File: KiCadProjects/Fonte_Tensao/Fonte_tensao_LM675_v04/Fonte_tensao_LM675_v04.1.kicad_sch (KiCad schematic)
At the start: 33 parts, among them J1 Barrel_Jack, J1 alimentacao analogica, J2 sinais analogicos, J3 comunicacao / sinais digitais, U1 L7809, U2 LM7909_TO220, U3 LM675, U4 L7805, U5 L7905, U6 LM1117T-3.3

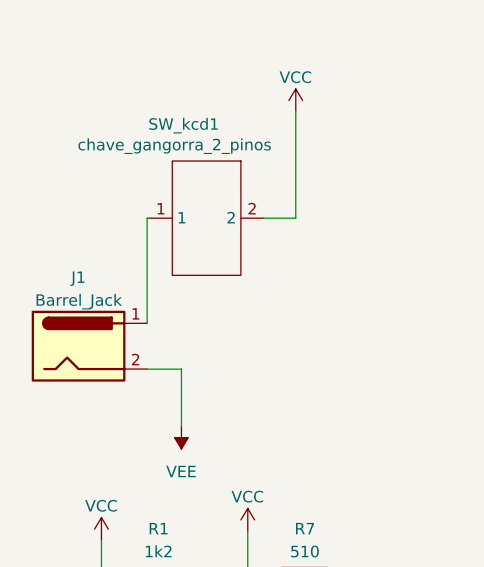
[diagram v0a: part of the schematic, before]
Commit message: correcao numeracao
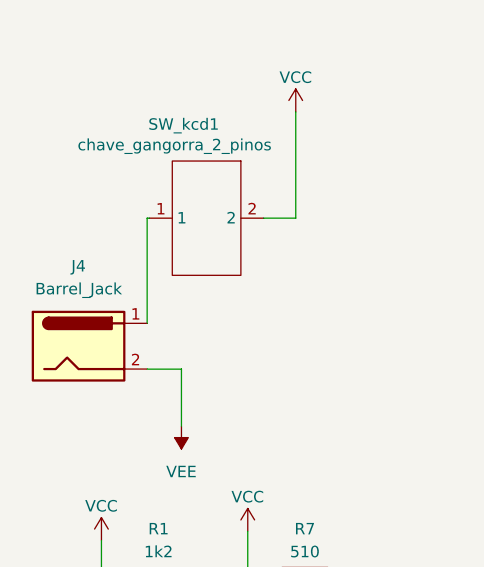
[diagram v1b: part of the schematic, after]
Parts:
- renumbered J1 to J4
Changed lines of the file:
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@@
   (symbol (lib_id "Connector:Barrel_Jack") (at 24.13 114.3 0) (unit 1)
     (in_bom yes) (on_board yes) (dnp no) (fields_autoplaced)
-    (property "Reference" "J1" (at 24.13 106.68 0)
+    (property "Reference" "J4" (at 24.13 105.41 0)
       (effects (font (size 1.27 1.27)))
     )
-    (property "Value" "Barrel_Jack" (at 24.13 109.22 0)
+    (property "Value" "Barrel_Jack" (at 24.13 107.95 0)
       (effects (font (size 1.27 1.27)))
     )
@@
       (project "Fonte_tensao_LM675_v04.1"
         (path "/f0ff92cf-26e5-4ab9-977d-5f9689e8a5d0"
-          (reference "J1") (unit 1)
+          (reference "J4") (unit 1)
         )
       )
